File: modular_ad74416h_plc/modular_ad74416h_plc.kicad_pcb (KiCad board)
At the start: 2 copper layers, 45.7 x 2.5 mm, 7 parts

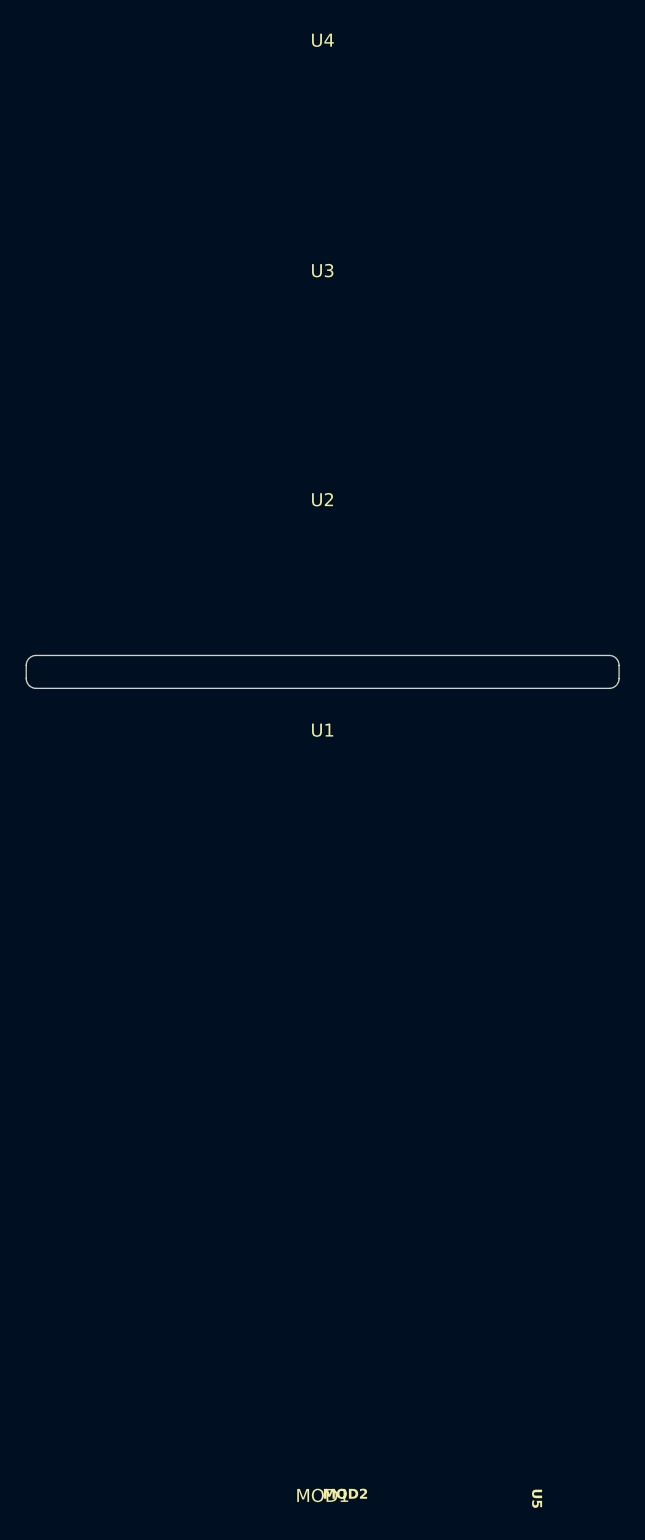
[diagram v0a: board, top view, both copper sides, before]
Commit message: backup
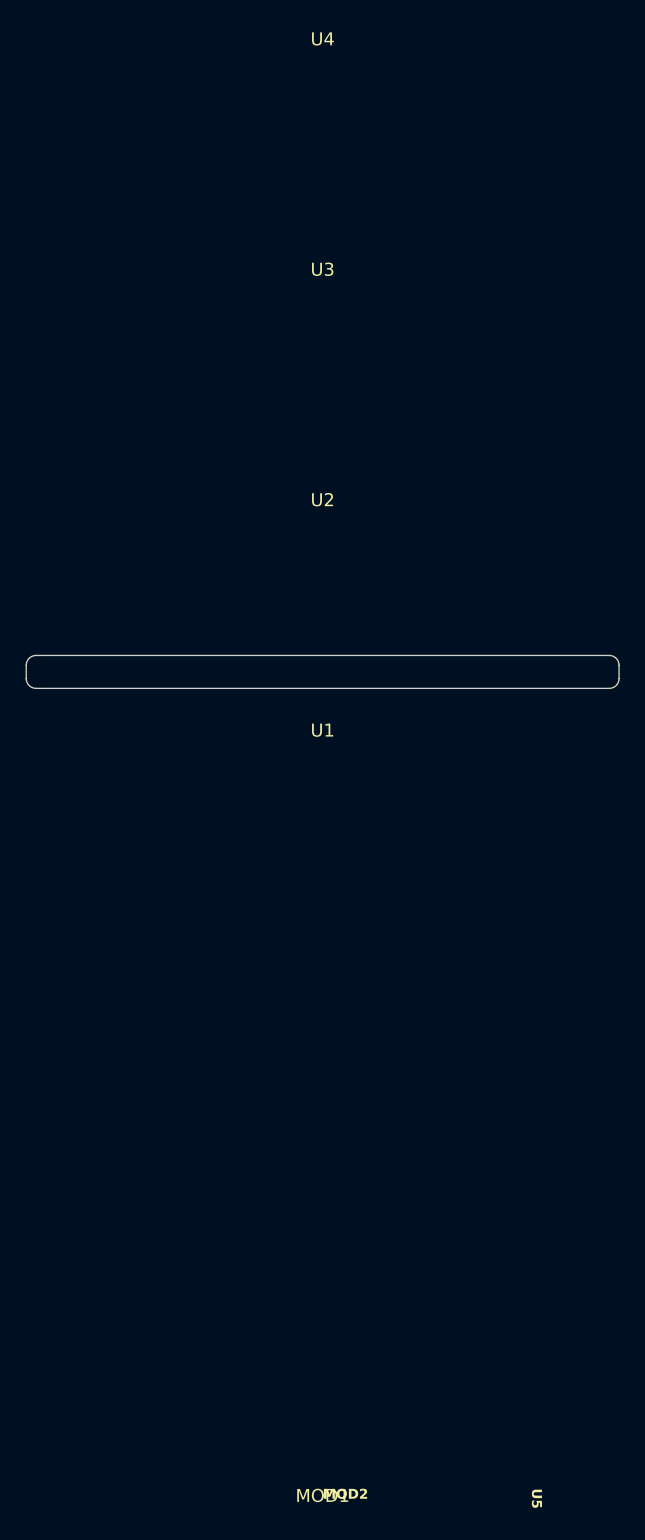
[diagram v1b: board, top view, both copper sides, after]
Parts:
- moved U3 0.10 mm to (193.8, 113.7)
- moved U4 0.10 mm to (193.8, 95.9)
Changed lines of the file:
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@@
 		(model "${KICAD9_3D_MODELS_VAULT}/3D_models/modules/minimal_ad74416h.step"
 			(offset
-				(xyz 0 0 6.985)
+				(xyz 0 0 4.318)
 			)
 			(scale
@@
 	(footprint "modules_footprints:minimal_ad74416h"
 		(layer "F.Cu")
-		(at 193.8274 96.012)
+		(at 193.8274 95.90786)
 		(property "Reference" "U4"
 			(at 0 -0.5 0)
@@
 		(model "${KICAD9_3D_MODELS_VAULT}/3D_models/modules/minimal_ad74416h.step"
 			(offset
-				(xyz 0 0 23.495)
+				(xyz 0 0 15.748)
 			)
 			(scale
@@
 	(footprint "modules_footprints:minimal_ad74416h"
 		(layer "F.Cu")
-		(at 193.8274 113.792)
+		(at 193.8274 113.68786)
 		(property "Reference" "U3"
 			(at 0 -0.5 0)
@@
 		(model "${KICAD9_3D_MODELS_VAULT}/3D_models/modules/minimal_ad74416h.step"
 			(offset
-				(xyz 0 0 15.24)
+				(xyz 0 0 10.033)
 			)
 			(scale
@@
 	(footprint "modules_footprints:minimal_adpl76030"
 		(layer "F.Cu")
-		(at 210.3501 207.2259 -90)
+		(at 210.3374 207.2259 -90)
 		(property "Reference" "U5"
 			(at 0 0 270)
